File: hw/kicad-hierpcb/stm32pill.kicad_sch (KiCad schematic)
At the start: 12 parts, among them U2 STM32F103C8T6

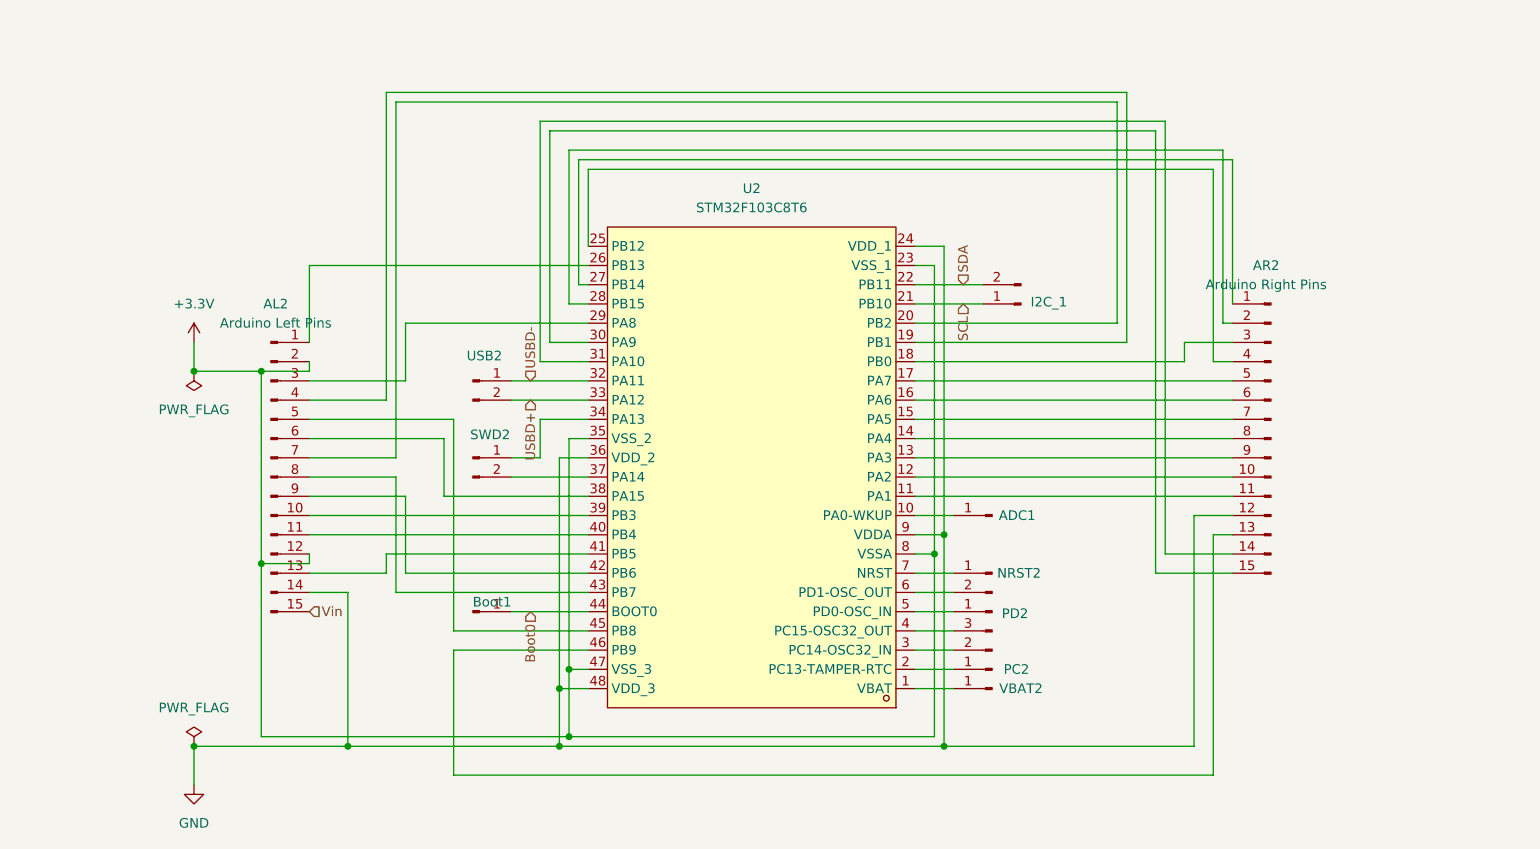
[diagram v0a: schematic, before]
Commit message: ide stm
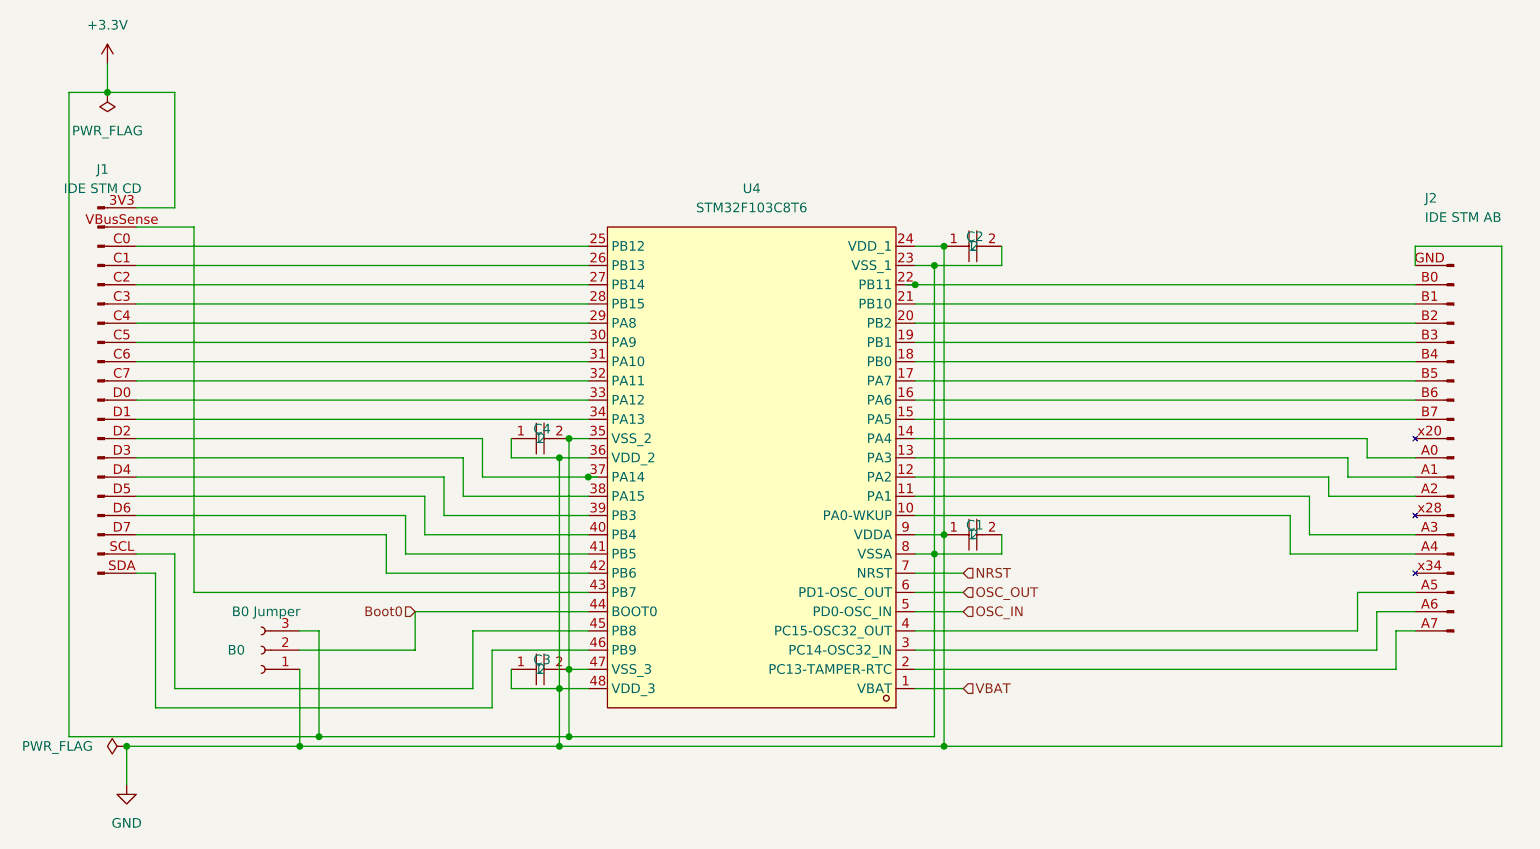
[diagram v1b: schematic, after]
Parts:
- removed ADC1: ADC0, base:PTH, symbol Connector:Conn_01x01_Pin
- removed AL2: Arduino Left Pins, Connector_PinHeader_2.54mm:PinHeader_1x15_P2.54mm_Vertical, symbol Connector:Conn_01x15_Pin
- removed AR2: Arduino Right Pins, Connector_PinHeader_2.54mm:PinHeader_1x15_P2.54mm_Vertical, symbol Connector:Conn_01x15_Pin
- removed Boot1: Boot0, base:PTH, symbol Connector:Conn_01x01_Pin
- removed I2C_1: I2C_2, Connector_PinHeader_2.54mm:PinHeader_1x02_P2.54mm_Vertical, symbol Connector:Conn_01x02_Pin
- removed NRST2: NRST, base:PTH, symbol Connector:Conn_01x01_Pin
- removed PC2: PC, Connector_PinHeader_2.54mm:PinHeader_1x03_P2.54mm_Vertical, symbol Connector:Conn_01x03_Pin
- removed PD2: PD, Connector_PinHeader_2.54mm:PinHeader_1x02_P2.54mm_Vertical, symbol Connector:Conn_01x02_Pin
- removed SWD2: SWD, Connector_PinHeader_2.54mm:PinHeader_1x02_P2.54mm_Vertical, symbol Connector:Conn_01x02_Pin
- removed USB2: USB, Connector_PinHeader_2.54mm:PinHeader_1x02_P2.54mm_Vertical, symbol Connector:Conn_01x02_Pin
- removed VBAT2: VBAT, base:PTH, symbol Connector:Conn_01x01_Pin
- added B0: B0 Jumper, base:3x PTH 1.7mm, symbol Connector:Conn_01x03_Socket
- added C1, C2, C3, C4: CL21B103KBANNNC, jlcpcb:C0805, symbol jlcpcb:Capacitor 10nF CL21B103KBANNNC
- added J1: IDE STM CD, ribbon:IDE STM CD, symbol ribbon:IDE STM CD
- added J2: IDE STM AB, ribbon:IDE STM AB, symbol ribbon:IDE STM AB
- renumbered U2 to U4
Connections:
- net +3.3V: now also B0.3 (Pin_3), C1.2, C2.2, C3.2, C4.2, J1.3V3 (IDE1_STM23)
- net Boot0: now also B0.2 (Pin_2)
- net GND: now also B0.1 (Pin_1), C1.1, C2.1, C3.1, C4.1, J2.GND (IDE2_STM24)
- net VBAT: now reaches U4.1 (VBAT)
- net at U4.10 (PA0-WKUP): now also J2.A4 (IDE32_STM10)
- net at U4.11 (PA1): now also J2.A3 (IDE30_STM11)
- net at U4.12 (PA2): now also J2.A2 (IDE26_STM12)
- net at U4.13 (PA3): now also J2.A1 (IDE24_STM13)
- net at U4.14 (PA4): now also J2.A0 (IDE22_STM14)
- net at U4.15 (PA5): now also J2.B7 (IDE18_STM15)
- net at U4.16 (PA6): now also J2.B6 (IDE16_STM16)
- net at U4.17 (PA7): now also J2.B5 (IDE14_STM17)
- net at U4.18 (PB0): now also J2.B4 (IDE12_STM18)
- net at U4.19 (PB1): now also J2.B3 (IDE10_STM19)
- net at U4.2 (PC13-TAMPER-RTC): now also J2.A7 (IDE40_STM2)
- net at U4.20 (PB2): now also J2.B2 (IDE8_STM20)
- net at U4.25 (PB12): now also J1.C0 (IDE5_STM25)
- net at U4.26 (PB13): now also J1.C1 (IDE7_STM26)
- net at U4.27 (PB14): now also J1.C2 (IDE9_STM27)
- net at U4.28 (PB15): now also J1.C3 (IDE11_STM28)
- net at U4.29 (PA8): now also J1.C4 (IDE13_STM29)
- net at U4.3 (PC14-OSC32_IN): now also J2.A6 (IDE38_STM3)
- net at U4.30 (PA9): now also J1.C5 (IDE15_STM30)
- net at U4.31 (PA10): now also J1.C6 (IDE17_STM31)
- net at U4.34 (PA13): now also J1.D1 (IDE23_STM34)
- net at U4.37 (PA14): now also J1.D2 (IDE25_STM37)
- net at U4.38 (PA15): now also J1.D3 (IDE27_STM38)
- net at U4.39 (PB3): now also J1.D4 (IDE29_STM39)
- net at U4.4 (PC15-OSC32_OUT): now also J2.A5 (IDE36_STM4)
- net at U4.40 (PB4): now also J1.D5 (IDE31_STM40)
- net at U4.41 (PB5): now also J1.D6 (IDE33_STM41)
- net at U4.42 (PB6): now also J1.D7 (IDE35_STM42)
- net at U4.43 (PB7): now also J1.VBusSense (IDE3_STM43)
- net at U4.45 (PB8): now also J1.SCL (IDE37_STM45)
- net at U4.46 (PB9): now also J1.SDA (IDE39_STM46)
- net OSC_IN: now reaches U4.5 (PD0-OSC_IN)
- net OSC_OUT: now reaches U4.6 (PD1-OSC_OUT)
- net NRST: now reaches U4.7 (NRST)
- net SCL: no longer names the net of U4.21 (PB10)
- net SCL: now also J2.B1 (IDE6_STM21)
- net SDA: no longer names the net of U4.22 (PB11)
- net SDA: now also J2.B0 (IDE4_STM22)
- net USBD+: no longer names the net of U4.33 (PA12)
- net USBD+: now also J1.D0 (IDE21_STM33)
- net USBD-: no longer names the net of U4.32 (PA11)
- net USBD-: now also J1.C7 (IDE19_STM32)
